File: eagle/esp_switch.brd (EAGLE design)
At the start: 55 x 27 mm, 22 parts, among them IC1 LT1117-3.3V, X1 MKDSN1,5/3-5,08

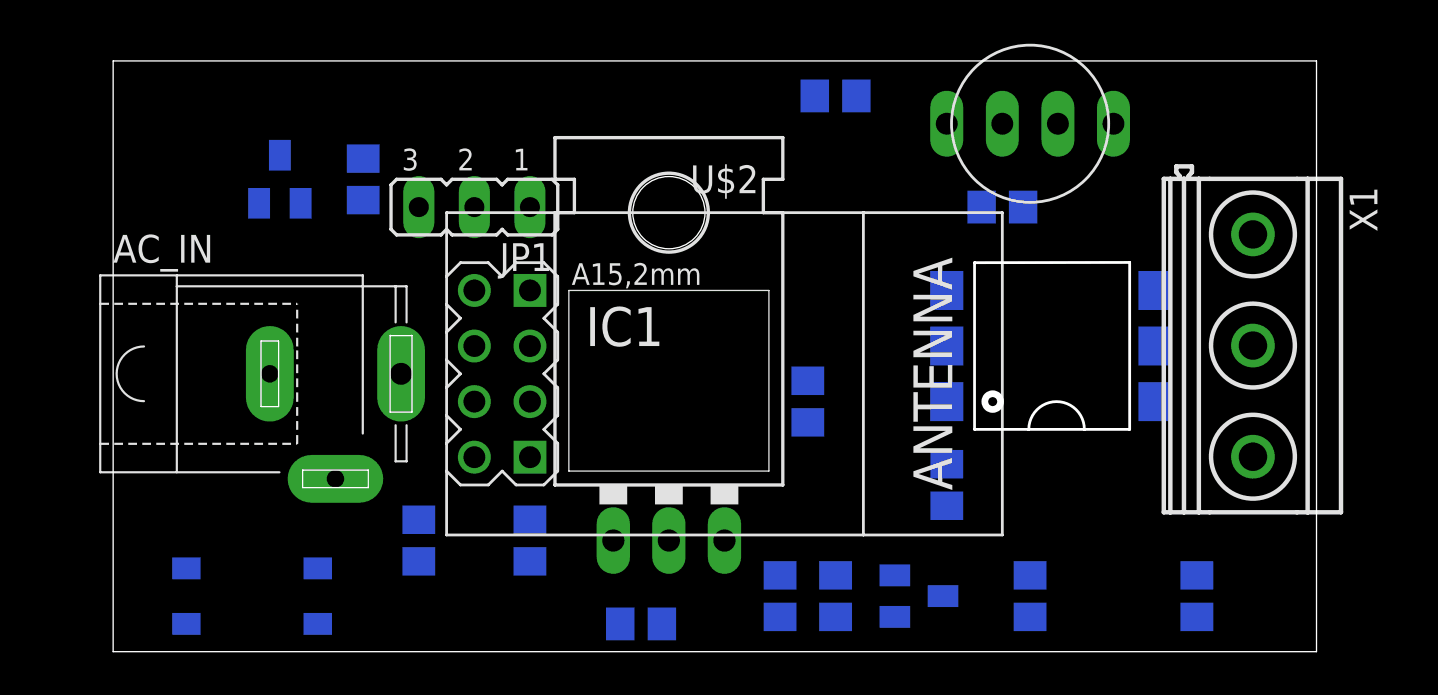
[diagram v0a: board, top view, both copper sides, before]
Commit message: brd modified2
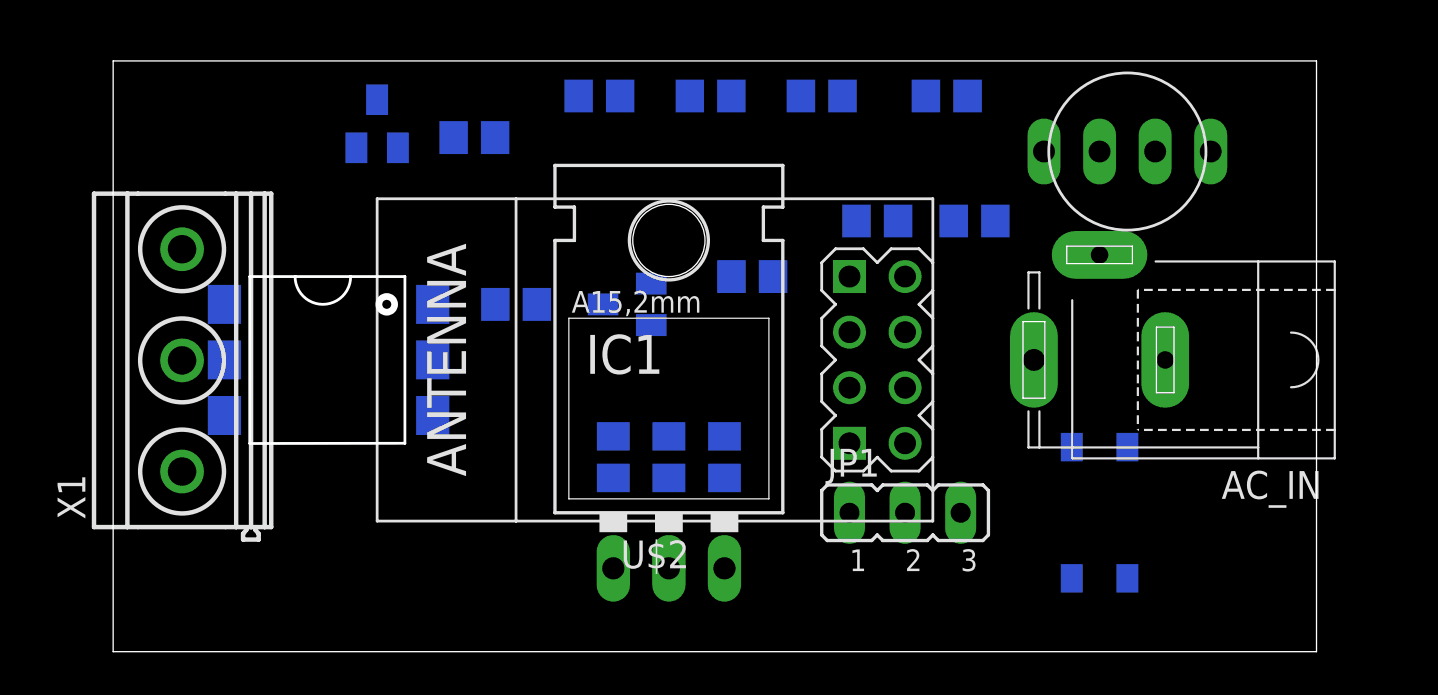
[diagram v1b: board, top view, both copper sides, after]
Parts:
- moved X1 49.1 mm to (3.17, 15.9), turned to 90 degrees
- moved D1 38.9 mm to (45.1, 6.35), turned to 0 degrees
- moved AC_IN 34.9 mm to (45.1, 13.3), turned to 180 degrees
- moved R3 24.8 mm to (32.4, 25.4), turned to 180 degrees
- moved R7 24.3 mm to (22.2, 25.4), turned to 0 degrees
- moved JP1 24.1 mm to (36.2, 6.35), turned to 0 degrees
- moved LH1500 23.9 mm to (14.6, 15.9), turned to 0 degrees
- moved R8 23.6 mm to (27.3, 25.4), turned to 0 degrees
- moved C1 22.5 mm to (27.9, 8.89), turned to 90 degrees
- moved R9 21.3 mm to (18.4, 15.9), turned to 180 degrees
- moved Q2 18.9 mm to (23.5, 15.9), turned to 270 degrees
- moved R1 16.7 mm to (29.2, 17.1), turned to 0 degrees
- moved C2 9.67 mm to (22.9, 8.89), turned to 90 degrees
- moved R2 8.84 mm to (34.9, 19.7), turned to 180 degrees
- moved R5 8.54 mm to (39.4, 19.7)
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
